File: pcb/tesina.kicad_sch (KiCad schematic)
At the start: 19 parts, among them J1 Conn_01x02_Male, J2 Conn_01x02_Male, J5 AMP2_IN, J6 AMP3_IN, J7 AMP2_OUT, J8 AMP3_OUT

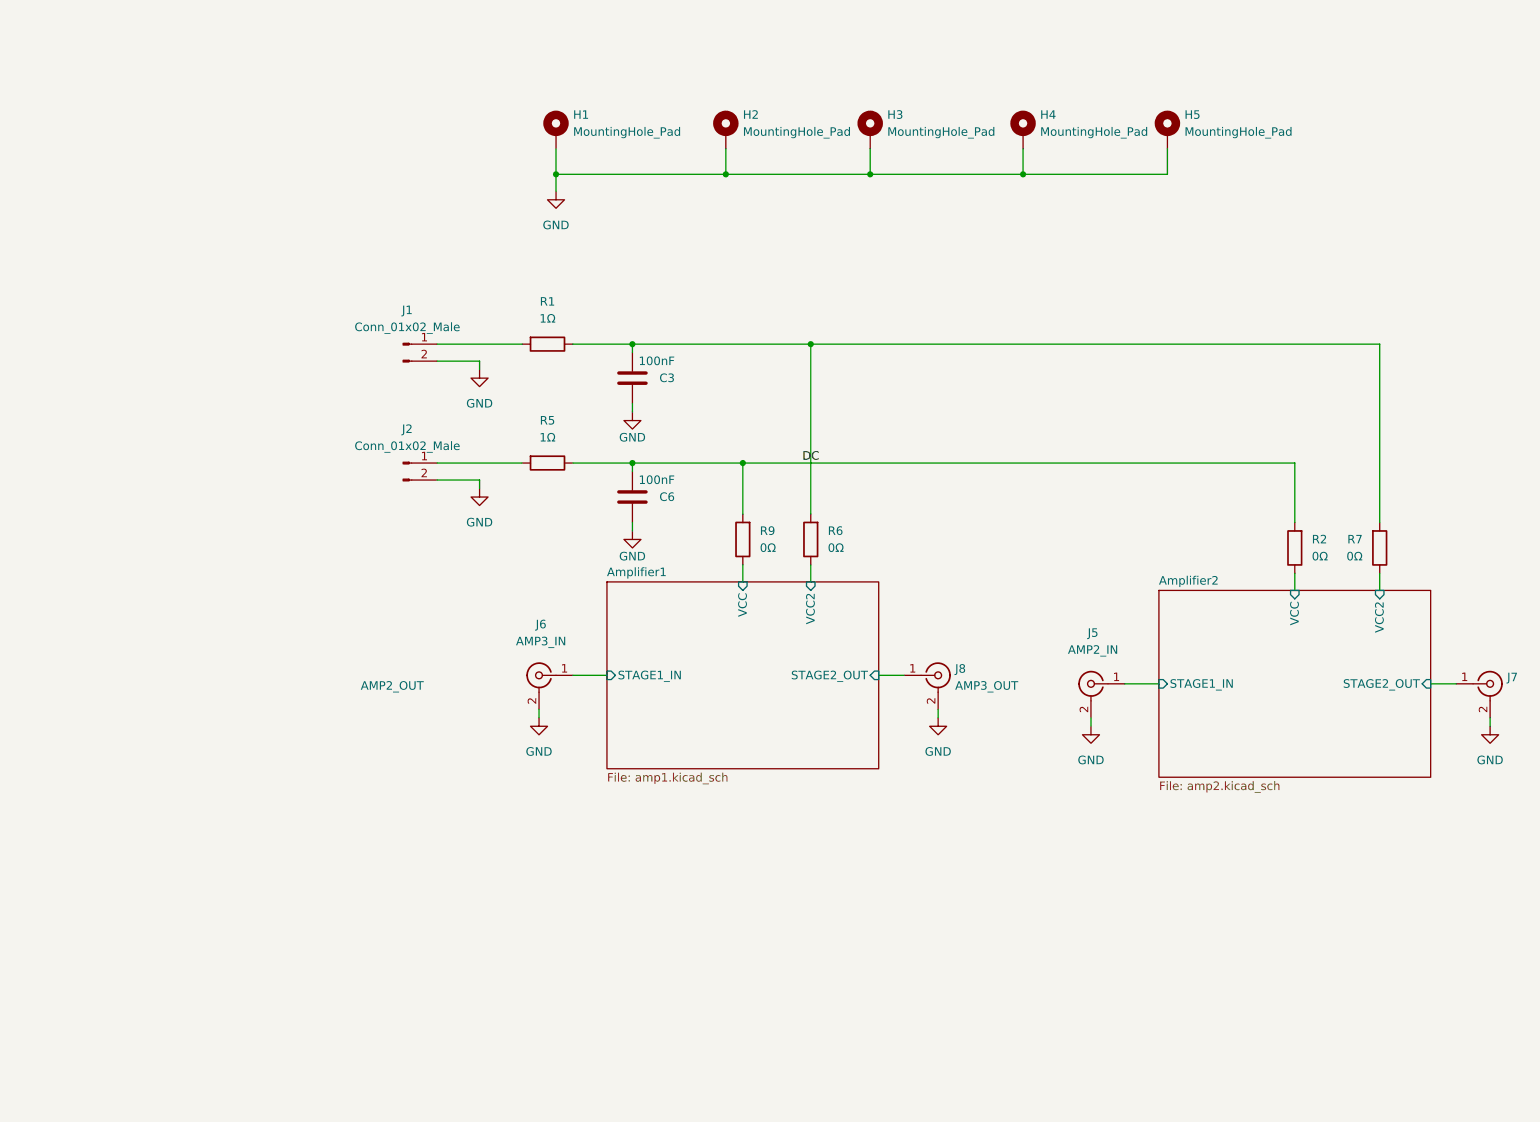
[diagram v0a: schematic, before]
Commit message: graduated
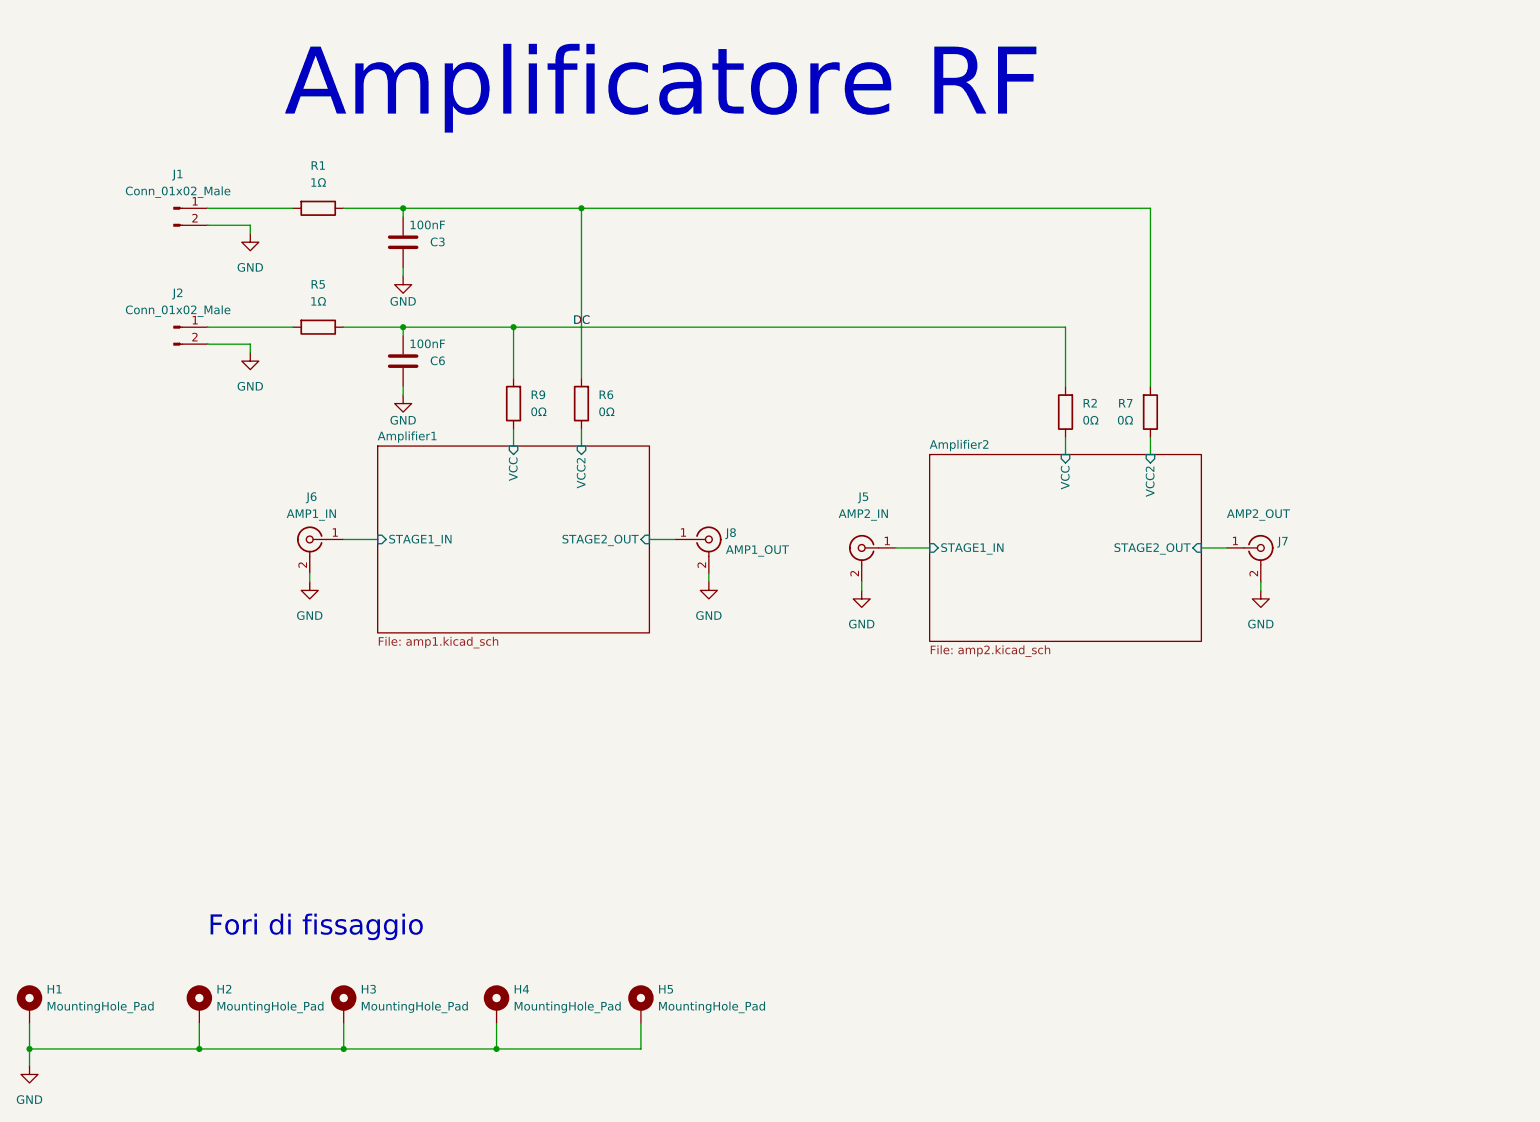
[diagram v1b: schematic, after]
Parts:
- J6: value AMP3_IN -> AMP1_IN
- J8: value AMP3_OUT -> AMP1_OUT
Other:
- note added: "Amplificatore RF"
- note added: "Fori di fissaggio"
- moved on the sheet: C3, C6, H1, H2, H3, H4, H5, J1, J2, J5, J6, J7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
